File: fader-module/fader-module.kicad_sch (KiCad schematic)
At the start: 33 parts, among them J1 Conn_1x05_Pin, J2 Conn_1x05_Socket, J7 Conn_01x06_Socket, SW1 1825910-6, SW2 1825910-6, U5 ATMEGA328P-AUR, U7 DRV8871DDAR

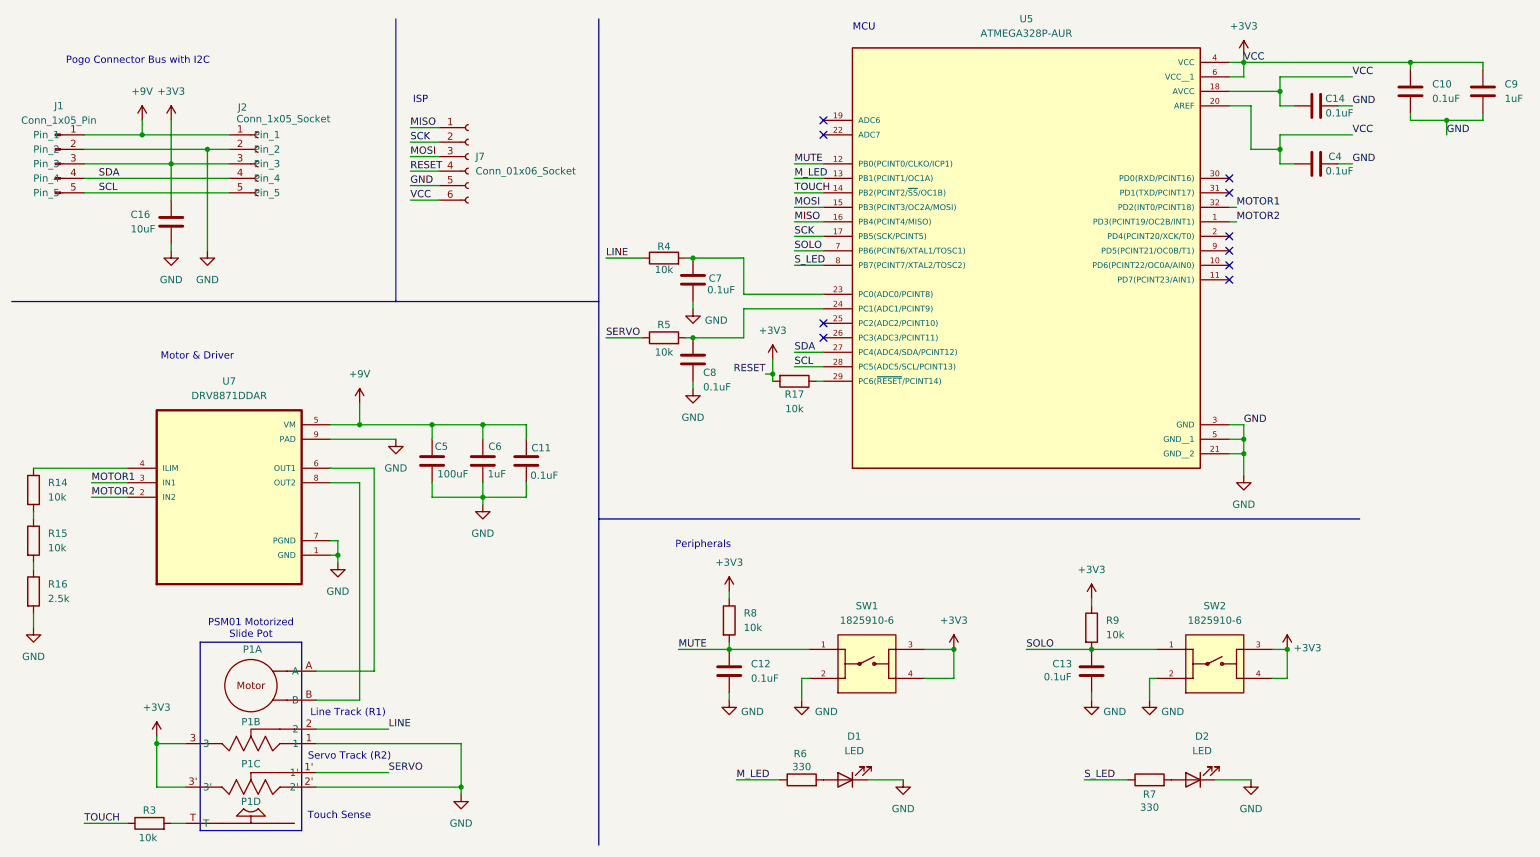
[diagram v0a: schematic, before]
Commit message: i will combust
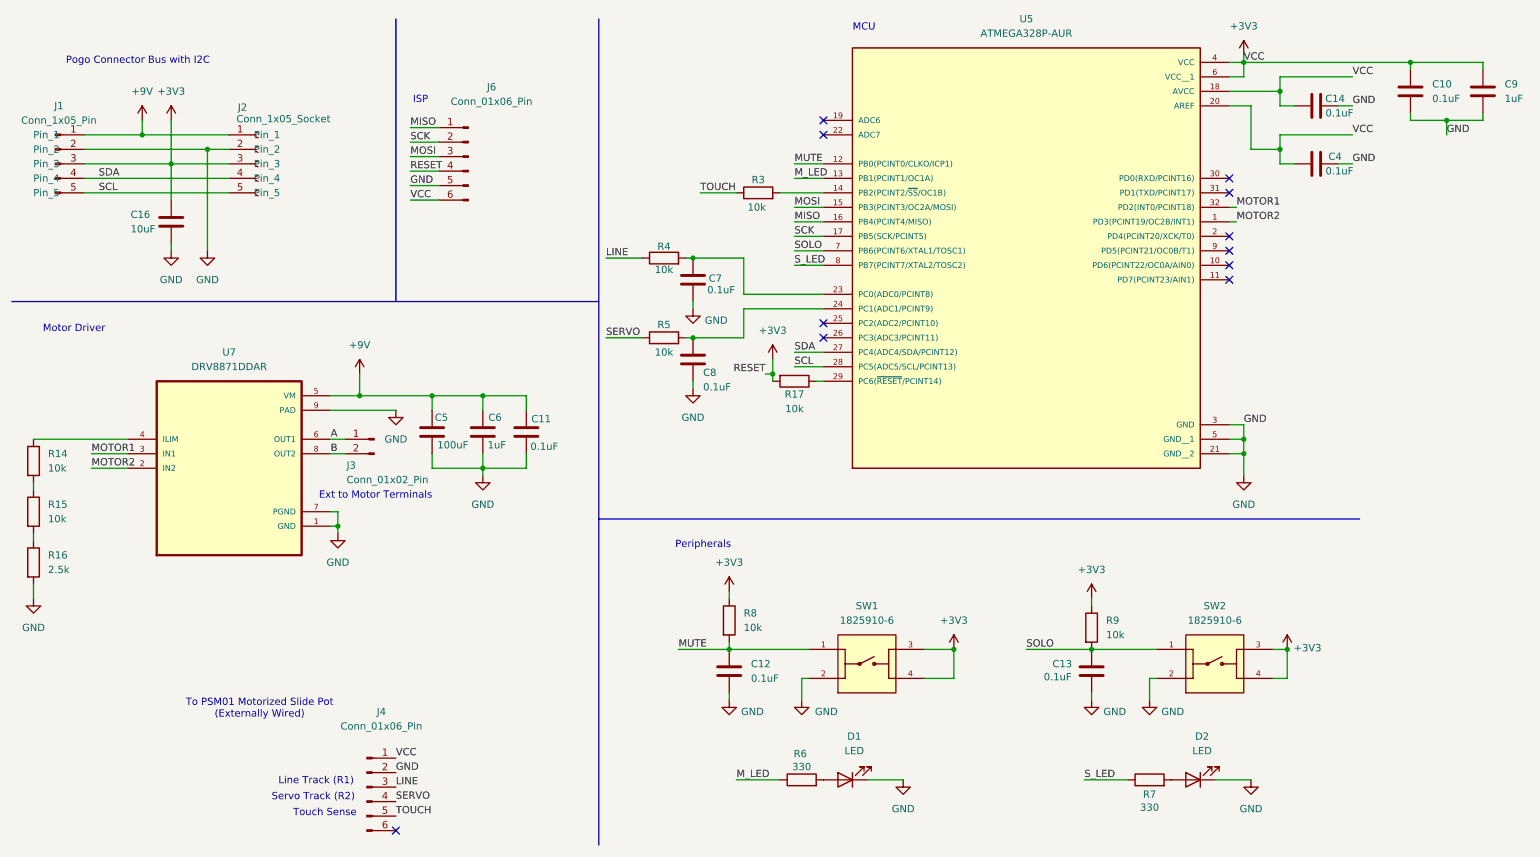
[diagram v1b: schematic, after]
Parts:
- removed J7: Conn_01x06_Socket, Connector_IDC:IDC-Header_2x03_P2.54mm_Vertical, symbol Connector:Conn_01x06_Socket
- removed P1: ~, PSM01:PSM01-081A_BRN, symbol PSM01:PSM01
- added J3: Conn_01x02_Pin, TerminalBlock_Phoenix:TerminalBlock_Phoenix_MKDS-1,5-2-5.08_1x02_P5.08mm_Horizontal, symbol Connector:Conn_01x02_Pin
- added J4, J6: Conn_01x06_Pin, Connector_IDC:IDC-Header_2x03_P2.54mm_Vertical, symbol Connector:Conn_01x06_Pin
- D1, D2: footprint LED_SMD:LED_0805_2012Metric_Pad1.15x1.40mm_HandSolder -> Connector_Molex:Molex_KK-254_AE-6410-02A_1x02_P2.54mm_Vertical
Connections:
- net +3V3: now also J4.1 (Pin_1), J6.4 (Pin_4), J6.6 (Pin_6)
- net GND: now also J4.2 (Pin_2), J6.5 (Pin_5)
- net LINE: now also J4.3 (Pin_3)
- net MISO: now also J6.1 (Pin_1)
- net MOSI: now also J6.3 (Pin_3)
- net SCK: now also J6.2 (Pin_2)
- net SERVO: now also J4.4 (Pin_4)
- net TOUCH: now also J4.5 (Pin_5); no longer U5.14 (PB2(PCINT2/~{SS}/OC1B))
- net A: now reaches U7.6 (OUT1)
- net A: now also J3.1 (Pin_1)
- net B: now reaches U7.8 (OUT2)
- net B: now also J3.2 (Pin_2)
- net at R3.2: now also U5.14 (PB2(PCINT2/~{SS}/OC1B))
- no-connect marks 10 -> 11
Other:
- note added: "Ext to Motor Terminals"
- note added: "Motor Driver"
- note added: "To PSM01 Motorized Slide Pot (Externally Wired)"
- note removed: "Motor & Driver"
- note removed: "PSM01 Motorized Slide Pot"
- moved on the sheet: C11, C5, C6, R14, R15, R16, R3, U7
